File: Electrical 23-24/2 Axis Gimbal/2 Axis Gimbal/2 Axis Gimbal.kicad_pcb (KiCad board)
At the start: 2 copper layers, 45 x 45 mm, 28 parts, among them IC1 BNO085, IC2 AP1086DL-13, J1 Conn_01x06_Socket, J2 Conn_01x06_Socket, U1 ATtiny404-SS

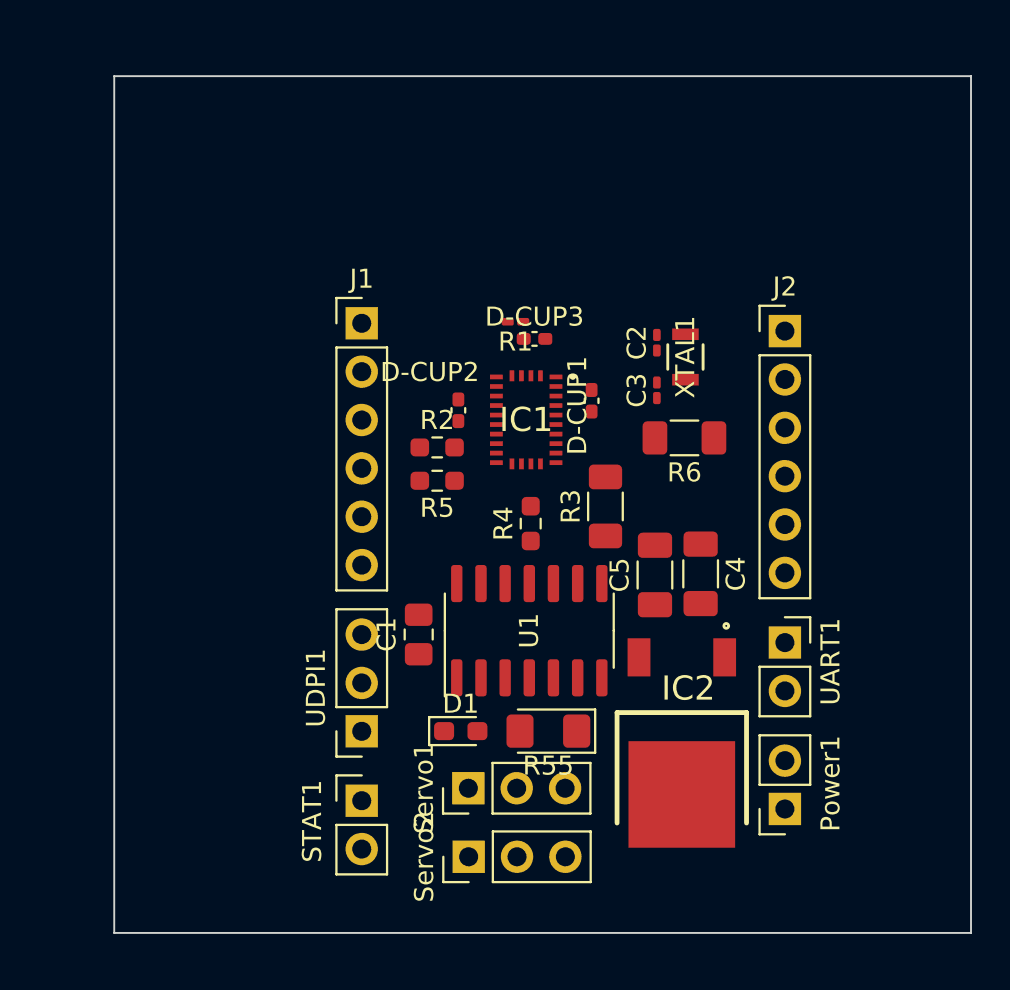
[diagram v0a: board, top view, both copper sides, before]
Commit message: Update 2 Axis Gimbal.kicad_pcb
Finished PCB
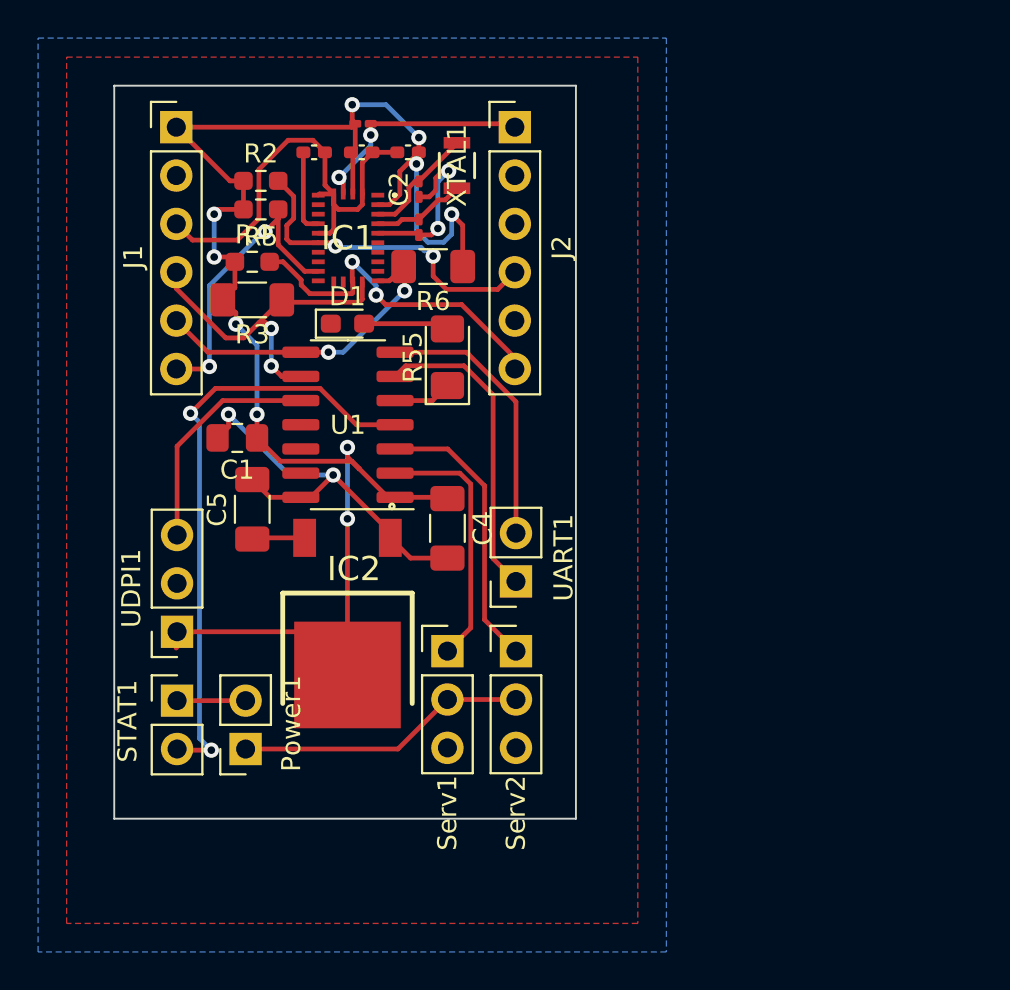
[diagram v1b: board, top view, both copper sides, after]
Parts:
- moved Power1 28.5 mm to (77.9, 107.3)
- moved D1 22.2 mm to (83.2, 85.0)
- moved R3 21.5 mm to (78.2, 83.8), turned to 180 degrees
- moved C5 21.4 mm to (78.2, 94.8)
- moved R55 20.3 mm to (88.5, 86.8), turned to 90 degrees
- moved R4 20.1 mm to (78.2, 81.8), turned to 0 degrees
- moved IC2 18.6 mm to (83.2, 105.0)
- moved J2 17.8 mm to (92.0, 74.7)
- moved R5 17.0 mm to (78.7, 79.0)
- moved R2 16.8 mm to (78.7, 77.5)
- moved D-CUP1 16.2 mm to (86.4, 76.0), turned to 180 degrees
- moved R6 16.0 mm to (87.8, 82.0)
- moved XTAL1 15.7 mm to (89.0, 76.7)
- moved D-CUP2 15.5 mm to (81.5, 76.0), turned to 180 degrees
- moved C3 15.2 mm to (87.0, 79.9)
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- renumbered Servo1 to Serv1, Servo2 to Serv2
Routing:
- net 3.3: track 0.00 -> 90.0 mm, vias 0 -> 10
- net GND: track 0.00 -> 58.8 mm, vias 0 -> 4
- net STAT: track 0.00 -> 32.0 mm, vias 0 -> 2
- net CSN: track 0.00 -> 18.4 mm, vias 0 -> 2
- net SCL: track 0.00 -> 18.1 mm, vias 0 -> 2
- net RST: track 0.00 -> 17.6 mm, vias 0 -> 2
- net SDA: track 0.00 -> 17.0 mm, vias 0 -> 2
- net RX: track 0.00 -> 16.3 mm
- net INT: track 0.00 -> 16.1 mm, vias 0 -> 2
- net +BATT: track 0.00 -> 15.3 mm
- net PWM 2: track 0.00 -> 14.9 mm
- net TX: track 0.00 -> 14.3 mm
- net PWM 1: track 0.00 -> 13.5 mm
- net UPDI: track 0.00 -> 12.2 mm
- net BOOTN: track 0.00 -> 12.1 mm, vias 0 -> 2
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- added copper zone on F.Cu, net (none)
- added copper zone on B.Cu, net GND
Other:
- board size 45 x 45 mm -> 24.2 x 38.5 mm
